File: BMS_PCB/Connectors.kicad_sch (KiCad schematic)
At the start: 7 parts, among them J1 Conn_01x37

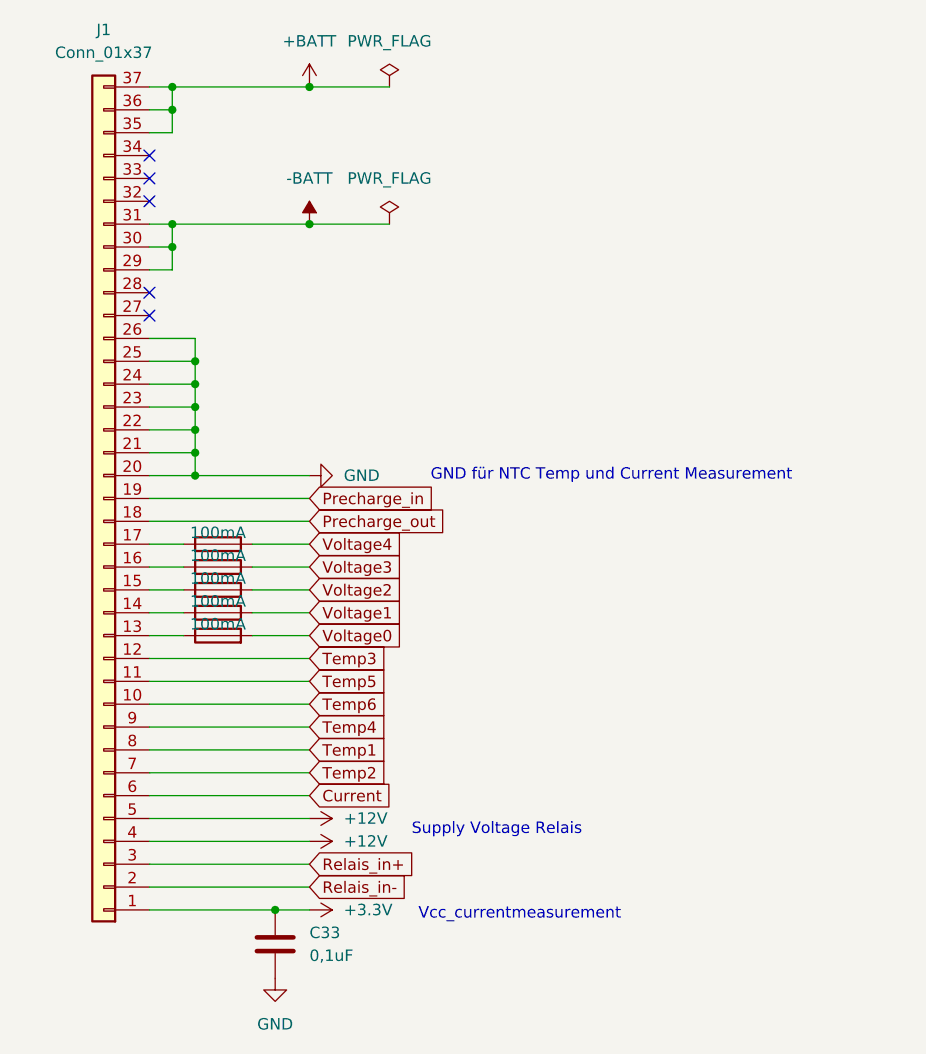
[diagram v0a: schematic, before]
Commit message: Freilaufdiode
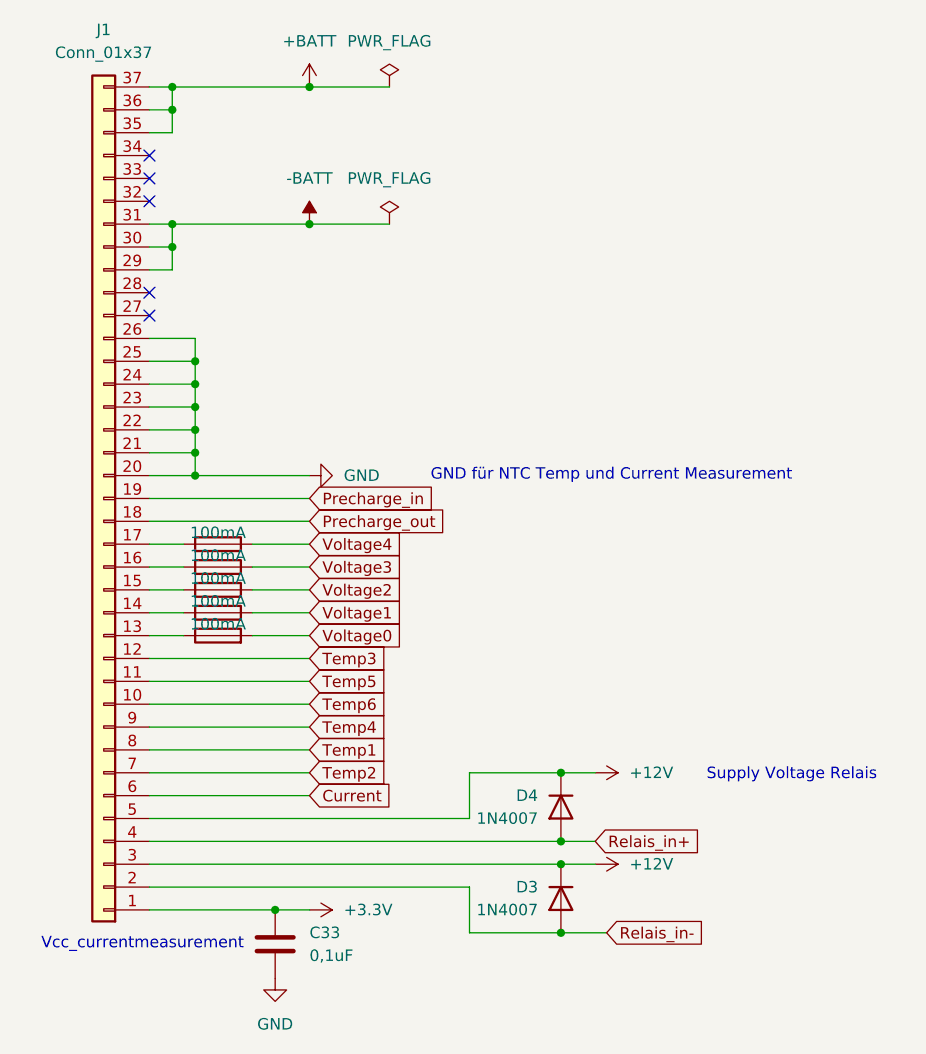
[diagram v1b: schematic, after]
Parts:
- added D3, D4: 1N4007, Diode_SMD:D_SMA, symbol Diode:1N4007
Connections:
- net +12V: now also J1.3 (Pin_3), D3.1 (K), D4.1 (K); no longer J1.4 (Pin_4)
- net Relais_in+: now also J1.4 (Pin_4), D4.2 (A); no longer J1.3 (Pin_3)
- net Relais_in-: now also D3.2 (A)
